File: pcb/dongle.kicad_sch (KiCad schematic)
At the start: 33 parts, among them J1 USB_A, J2 Conn_01x01_Pin, J3 Conn_01x01_Pin, J4 Conn_01x01_Pin, J5 Conn_01x01_Pin, SW1 SW_Push_45deg, U3 nRF52833_QDxx, Y1 Crystal_GND24, Y2 Crystal_Small

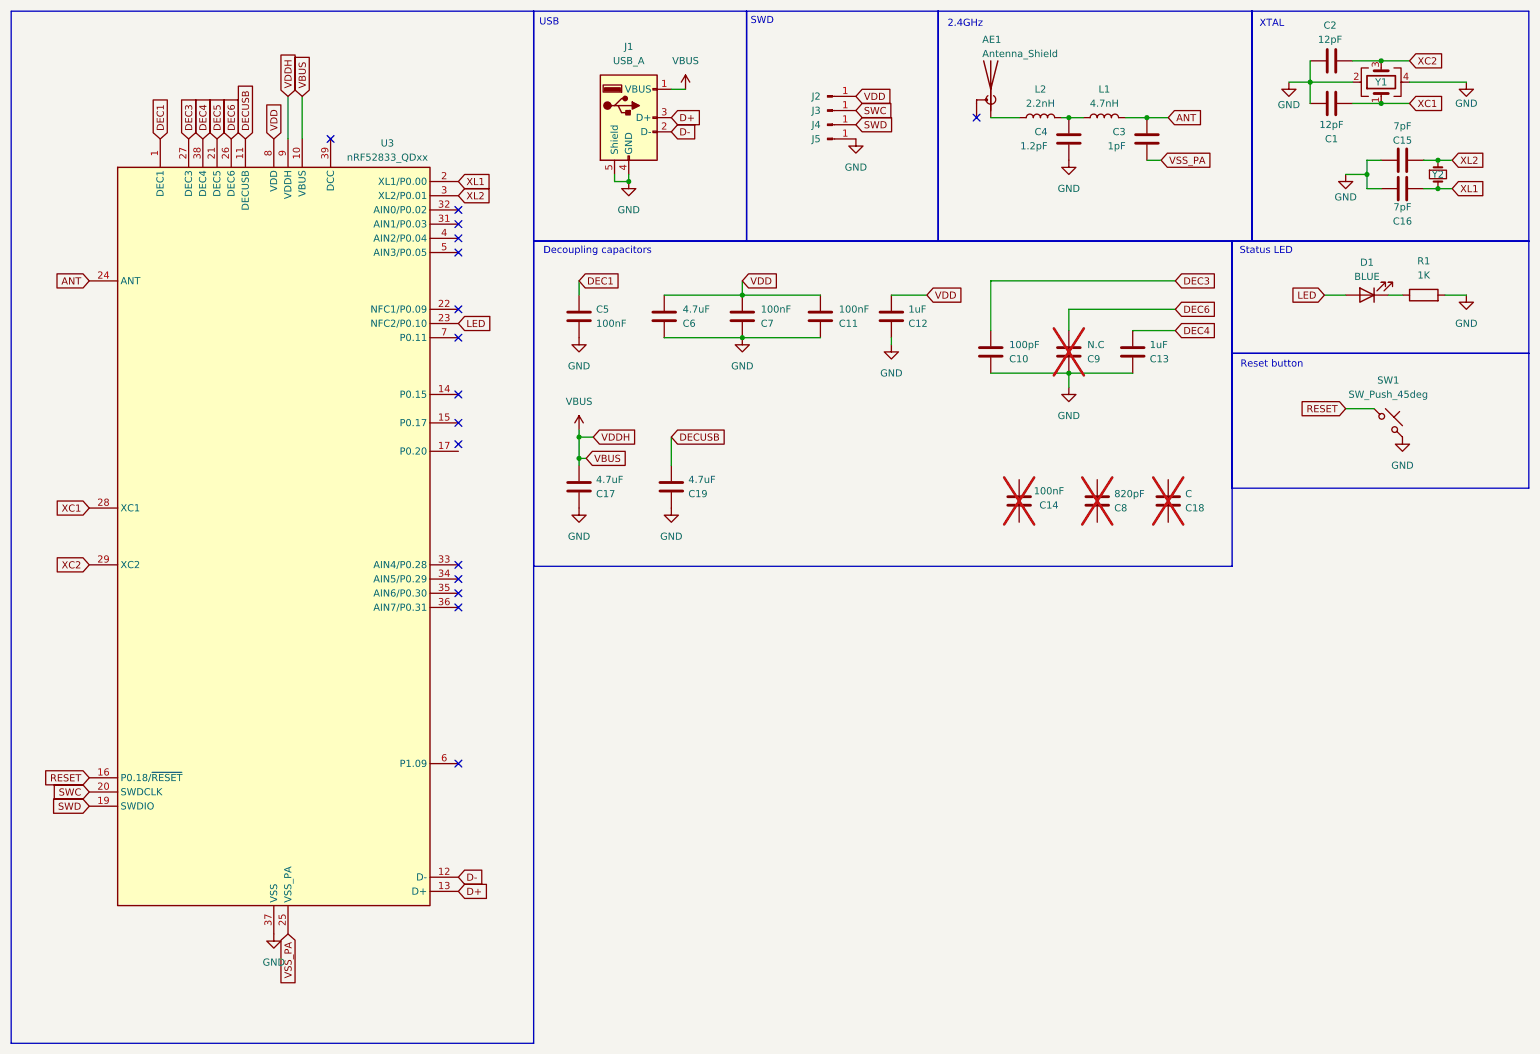
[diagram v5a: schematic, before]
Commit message: update pcb
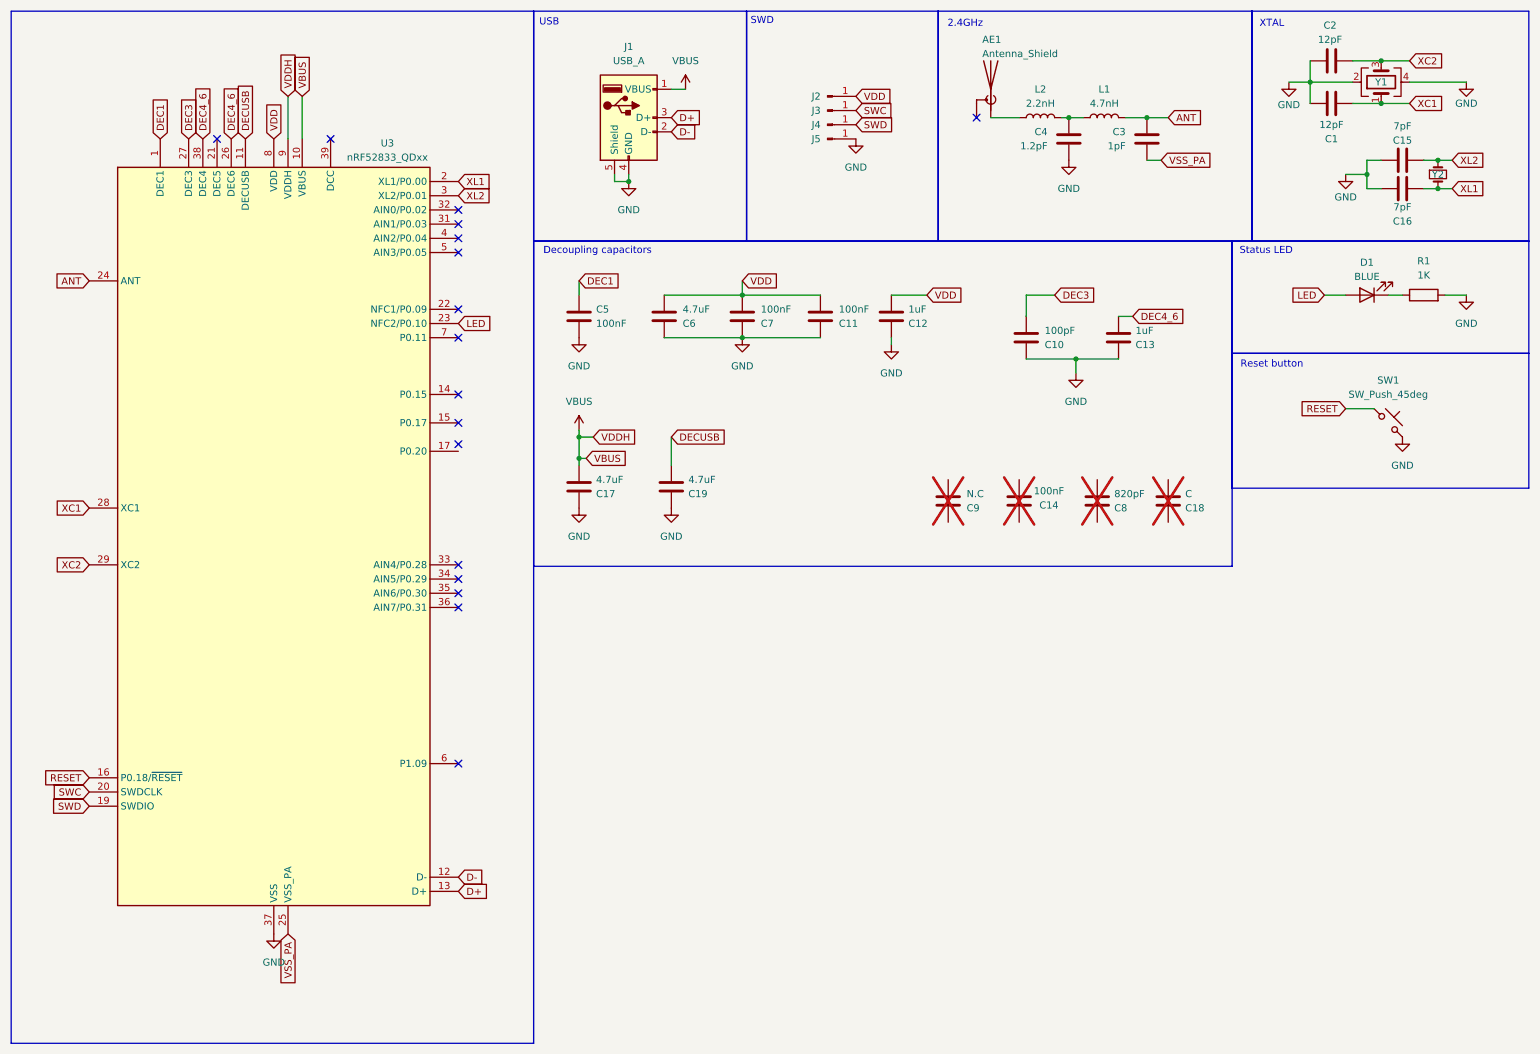
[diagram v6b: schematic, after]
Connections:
- net GND: no longer C9.1
- net DEC4 renamed DEC4_6
- net DEC4_6: now also U3.26 (DEC6)
- net DEC5: no longer names the net of U3.21 (DEC5)
- net DEC6: no longer names the net of C9.2
- net DEC6: no longer U3.26 (DEC6)
- no-connect marks 16 -> 17
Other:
- moved on the sheet: C10, C13, C9
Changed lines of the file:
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@@
 	)
 	(junction
+		(at 203.2 74.93)
+		(diameter 0)
+		(color 0 0 0 0)
+	)
+	(junction
 		(at 123.19 43.18)
 		(diameter 0)
@@
 	)
 	(junction
-		(at 201.93 77.47)
-		(diameter 0)
-		(color 0 0 0 0)
-	)
-	(junction
 		(at 257.81 29.21)
 		(diameter 0)
@@
 	)
 	(no_connect
+		(at 49.53 35.56)
+	)
+	(no_connect
 		(at 92.71 48.26)
 	)
@@
 	(wire
 		(pts
-			(xy 220.98 60.96) (xy 187.96 60.96)
+			(xy 199.39 63.5) (xy 194.31 63.5)
 		)
 		(stroke
@@
 	(wire
 		(pts
-			(xy 220.98 66.04) (xy 201.93 66.04)
-		)
-		(stroke
-			(width 0)
-			(type default)
-		)
-	)
-	(wire
-		(pts
 			(xy 245.11 25.4) (xy 252.73 25.4)
 		)
@@
 	(wire
 		(pts
-			(xy 220.98 69.85) (xy 213.36 69.85)
+			(xy 213.36 67.31) (xy 210.82 67.31)
 		)
 		(stroke
@@
 	(wire
 		(pts
-			(xy 187.96 77.47) (xy 201.93 77.47)
+			(xy 194.31 74.93) (xy 203.2 74.93)
 		)
 		(stroke
@@
 	(wire
 		(pts
-			(xy 187.96 60.96) (xy 187.96 69.85)
+			(xy 194.31 63.5) (xy 194.31 67.31)
 		)
 		(stroke
@@
 	(wire
 		(pts
-			(xy 201.93 80.01) (xy 201.93 77.47)
+			(xy 203.2 77.47) (xy 203.2 74.93)
 		)
 		(stroke
@@
 	(wire
 		(pts
-			(xy 201.93 66.04) (xy 201.93 69.85)
+			(xy 255.27 41.91) (xy 255.27 44.45)
 		)
 		(stroke
@@
 	(wire
 		(pts
-			(xy 255.27 41.91) (xy 255.27 44.45)
+			(xy 64.77 27.94) (xy 64.77 35.56)
 		)
 		(stroke
@@
 	(wire
 		(pts
-			(xy 64.77 27.94) (xy 64.77 35.56)
+			(xy 114.3 60.96) (xy 114.3 63.5)
 		)
 		(stroke
@@
 	(wire
 		(pts
-			(xy 114.3 60.96) (xy 114.3 63.5)
+			(xy 251.46 63.5) (xy 247.65 63.5)
 		)
 		(stroke
@@
 	(wire
 		(pts
-			(xy 251.46 63.5) (xy 247.65 63.5)
+			(xy 245.11 25.4) (xy 245.11 29.21)
 		)
 		(stroke
@@
 	(wire
 		(pts
-			(xy 245.11 25.4) (xy 245.11 29.21)
+			(xy 203.2 74.93) (xy 210.82 74.93)
 		)
 		(stroke
@@
 	(wire
 		(pts
-			(xy 201.93 77.47) (xy 213.36 77.47)
-		)
-		(stroke
-			(width 0)
-			(type default)
-		)
-	)
-	(wire
-		(pts
 			(xy 245.11 21.59) (xy 245.11 25.4)
 		)
@@
 		)
 	)
-	(global_label "DEC5"
-		(shape input)
-		(at 49.53 35.56 90)
-		(fields_autoplaced yes)
-		(effects
-			(font
-				(size 1.27 1.27)
-			)
-			(justify left)
-		)
-		(property "Intersheetrefs" "${INTERSHEET_REFS}"
-			(at 49.53 27.6763 90)
-			(effects
-				(font
-					(size 1.27 1.27)
-				)
-				(justify left)
-				(hide yes)
-			)
-		)
-	)
 	(global_label "DEC1"
 		(shape input)
@@
 		)
 	)
-	(global_label "DEC6"
-		(shape input)
-		(at 220.98 66.04 0)
-		(fields_autoplaced yes)
-		(effects
-			(font
-				(size 1.27 1.27)
-			)
-			(justify left)
-		)
-		(property "Intersheetrefs" "${INTERSHEET_REFS}"
-			(at 228.8637 66.04 0)
-			(effects
-				(font
-					(size 1.27 1.27)
-				)
-				(justify left)
-				(hide yes)
-			)
-		)
-	)
 	(global_label "LED"
 		(shape input)
@@
 	(global_label "DEC3"
 		(shape input)
-		(at 220.98 60.96 0)
+		(at 199.39 63.5 0)
 		(fields_autoplaced yes)
 		(effects
@@
 		)
 		(property "Intersheetrefs" "${INTERSHEET_REFS}"
-			(at 228.8637 60.96 0)
+			(at 207.2737 63.5 0)
 			(effects
 				(font
@@
 		)
 	)
-	(global_label "DEC4"
+	(global_label "DEC4_6"
 		(shape input)
 		(at 46.99 35.56 90)
@@
 		)
 		(property "Intersheetrefs" "${INTERSHEET_REFS}"
-			(at 46.99 27.6763 90)
+			(at 46.99 25.4992 90)
+			(effects
+				(font
+					(size 1.27 1.27)
+				)
+				(justify left)
+				(hide yes)
+			)
+		)
+	)
+	(global_label "DEC4_6"
+		(shape input)
+		(at 213.36 67.31 0)
+		(fields_autoplaced yes)
+		(effects
+			(font
+				(size 1.27 1.27)
+			)
+			(justify left)
+		)
+		(property "Intersheetrefs" "${INTERSHEET_REFS}"
+			(at 223.4208 67.31 0)
 			(effects
 				(font
@@
 		)
 	)
-	(global_label "DEC6"
+	(global_label "DEC4_6"
 		(shape input)
 		(at 52.07 35.56 90)
@@
 		)
 		(property "Intersheetrefs" "${INTERSHEET_REFS}"
-			(at 52.07 27.6763 90)
+			(at 52.07 25.4992 90)
 			(effects
 				(font
@@
 		)
 	)
-	(global_label "DEC4"
-		(shape input)
-		(at 220.98 69.85 0)
-		(fields_autoplaced yes)
-		(effects
-			(font
-				(size 1.27 1.27)
-			)
-			(justify left)
-		)
-		(property "Intersheetrefs" "${INTERSHEET_REFS}"
-			(at 228.8637 69.85 0)
-			(effects
-				(font
-					(size 1.27 1.27)
-				)
-				(justify left)
-				(hide yes)
-			)
-		)
-	)
 	(global_label "SWD"
 		(shape input)
@@
 	(symbol
 		(lib_id "Library:GND")
-		(at 201.93 80.01 0)
+		(at 203.2 77.47 0)
 		(unit 1)
 		(exclude_from_sim no)
@@
 		(fields_autoplaced yes)
 		(property "Reference" "#PWR08"
-			(at 201.93 86.36 0)
+			(at 203.2 83.82 0)
 			(effects
 				(font
@@
 		)
 		(property "Value" "GND"
-			(at 201.93 85.09 0)
+			(at 203.2 82.55 0)
 			(effects
 				(font
@@
 		)
 		(property "Footprint" ""
-			(at 201.93 80.01 0)
+			(at 203.2 77.47 0)
 			(effects
 				(font
@@
 		)
 		(property "Datasheet" ""
-			(at 201.93 80.01 0)
+			(at 203.2 77.47 0)
 			(effects
 				(font
@@
 		)
 		(property "Description" "Global ground symbol"
-			(at 201.93 89.408 0)
+			(at 203.2 86.868 0)
 			(effects
 				(font
@@
 	(symbol
 		(lib_id "PNCATEHO_lowair:C")
-		(at 187.96 73.66 0)
+		(at 194.31 71.12 0)
 		(mirror x)
 		(unit 1)
@@
 		(dnp no)
 		(property "Reference" "C10"
-			(at 191.262 74.93 0)
+			(at 197.612 72.39 0)
 			(effects
 				(font
@@
 		)
 		(property "Value" "100pF"
-			(at 191.262 72.39 0)
+			(at 197.612 69.85 0)
 			(effects
 				(font
@@
 		)
 		(property "Footprint" "dongle:C_0201_0603Metric"
-			(at 188.9252 69.85 0)
+			(at 195.2752 67.31 0)
 			(effects
 				(font
@@
 		)
 		(property "Datasheet" "~"
-			(at 187.96 73.66 0)
+			(at 194.31 71.12 0)
 			(effects
 				(font
@@
 		)
 		(property "Description" "Unpolarized capacitor"
-			(at 187.96 73.66 0)
+			(at 194.31 71.12 0)
 			(effects
 				(font
@@
 	(symbol
 		(lib_id "PNCATEHO_lowair:C")
-		(at 213.36 73.66 0)
+		(at 210.82 71.12 0)
 		(mirror x)
 		(unit 1)
@@
 		(dnp no)
 		(property "Reference" "C13"
-			(at 216.408 74.93 0)
+			(at 213.868 72.39 0)
 			(effects
 				(font
@@
 		)
 		(property "Value" "1uF"
-			(at 216.408 72.39 0)
+			(at 213.868 69.85 0)
 			(effects
 				(font
@@
 		)
 		(property "Footprint" "dongle:C_0402_1005Metric"
-			(at 214.3252 69.85 0)
+			(at 211.7852 67.31 0)
 			(effects
 				(font
@@
 		)
 		(property "Datasheet" "~"
-			(at 213.36 73.66 0)
+			(at 210.82 71.12 0)
 			(effects
 				(font
@@
 		)
 		(property "Description" "Unpolarized capacitor"
-			(at 213.36 73.66 0)
+			(at 210.82 71.12 0)
 			(effects
 				(font
@@
 	(symbol
 		(lib_id "PNCATEHO_lowair:C")
-		(at 201.93 73.66 0)
+		(at 180.34 100.33 0)
 		(mirror x)
 		(unit 1)
@@
 		(dnp yes)
 		(property "Reference" "C9"
-			(at 205.232 74.93 0)
+			(at 183.642 101.6 0)
 			(effects
 				(font
@@
 		)
 		(property "Value" "N.C"
-			(at 205.232 72.39 0)
+			(at 183.642 99.06 0)
 			(effects
 				(font
@@
 		)
 		(property "Footprint" "PNCATEHO_lowair:C_0201_0603Metric_Pad0.64x0.40mm_HandSolder"
-			(at 202.8952 69.85 0)
+			(at 181.3052 96.52 0)
 			(effects
 				(font
@@
 		)
 		(property "Datasheet" "~"
-			(at 201.93 73.66 0)
+			(at 180.34 100.33 0)
 			(effects
 				(font
@@
 		)
 		(property "Description" "Unpolarized capacitor"
-			(at 201.93 73.66 0)
+			(at 180.34 100.33 0)
 			(effects
 				(font
